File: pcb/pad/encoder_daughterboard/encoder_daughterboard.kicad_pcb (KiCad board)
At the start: 2 copper layers, 91.4 x 26.9 mm, 9 parts, among them J1 Conn_01x12, SW1 RotaryEncoder_Switch_MP, SW2 RotaryEncoder_Switch_MP, SW3 RotaryEncoder_Switch_MP

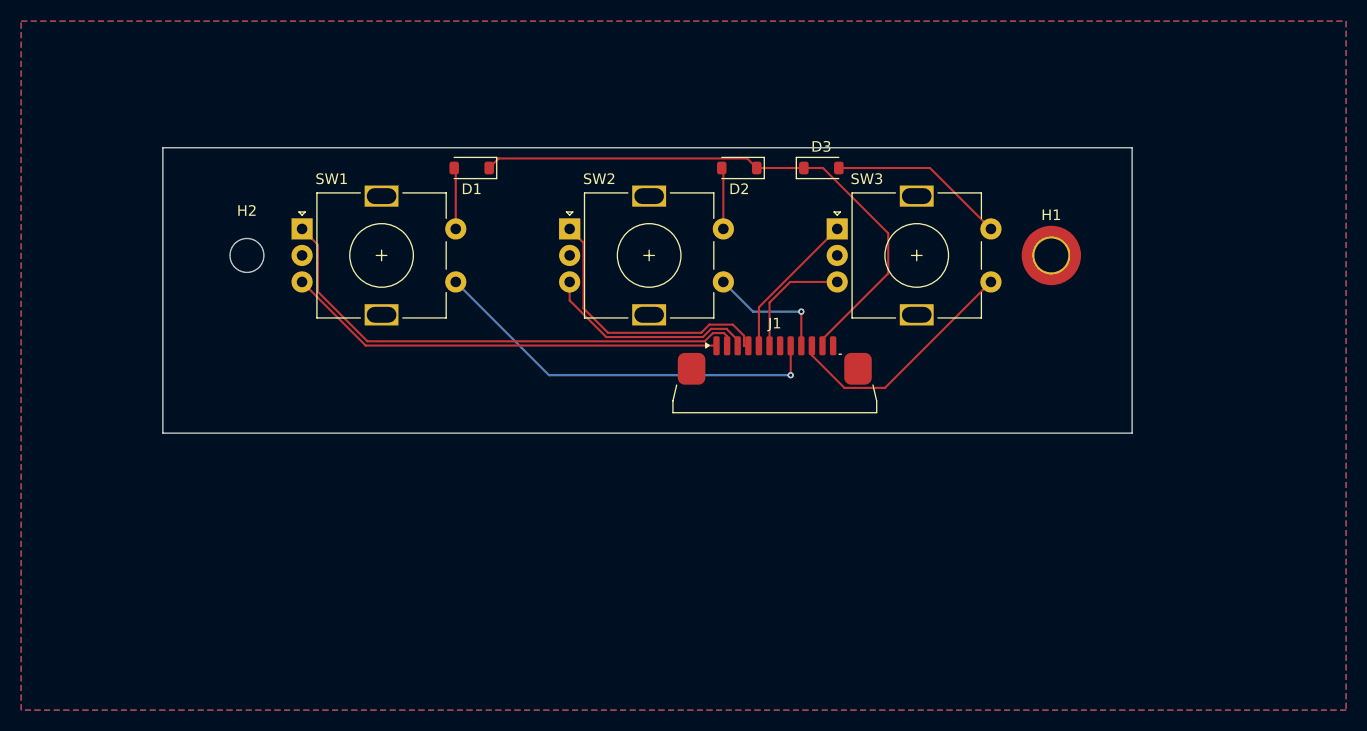
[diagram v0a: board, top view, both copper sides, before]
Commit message: Update encoder_daughterboard
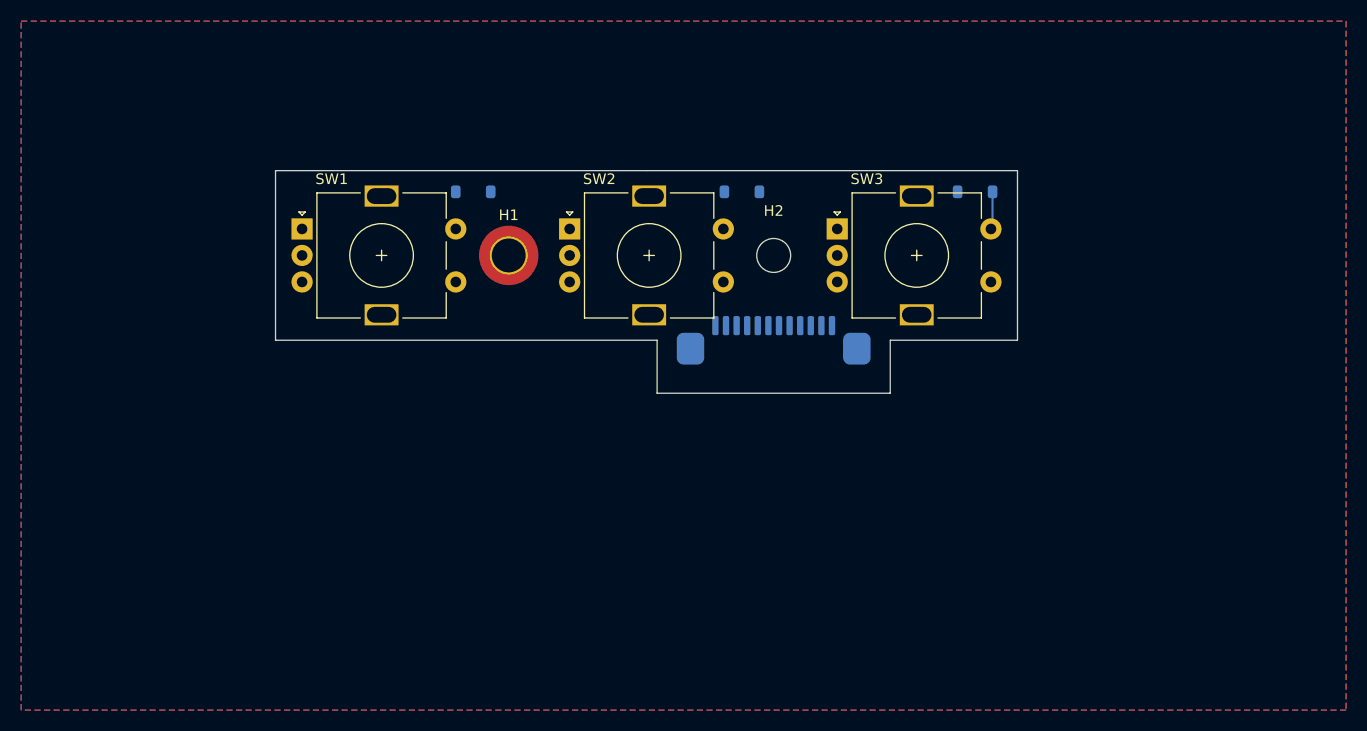
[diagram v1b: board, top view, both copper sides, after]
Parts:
- D1, D2, D3: moved to B.Cu
- J1: value Conn_01x12 -> AFA07-S12FCA-00; moved to B.Cu
- SW1, SW2, SW3: value RotaryEncoder_Switch_MP -> EC11E09244BS
- moved H1 51.2 mm to (95.2, 78.2)
- moved H2 49.7 mm to (120.2, 78.2)
- moved D3 14.7 mm to (139.2, 72.2)
- moved D2 2.26 mm to (117.2, 72.2)
- moved D1 2.25 mm to (91.9, 72.2)
- moved J1 1.90 mm to (120.2, 88.2), turned to 180 degrees
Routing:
- net BRow0: track 54.1 -> 0.00 mm
- net E0A: track 48.4 -> 0.00 mm
- net E0B: track 41.6 -> 0.00 mm
- net BCol0: track 38.0 -> 0.00 mm, vias 1 -> 0
- net E1A: track 26.2 -> 0.00 mm
- net BCol2: track 23.2 -> 0.00 mm
- net E1B: track 20.3 -> 0.00 mm
- net E2A: track 14.1 -> 0.00 mm
- net Net-(D3-A): track 16.7 -> 3.56 mm
- net BCol1: track 11.7 -> 0.00 mm, vias 1 -> 0
- net E2B: track 11.3 -> 0.00 mm
- net Net-(D2-A): track 5.81 -> 0.00 mm
- net Net-(D1-A): track 5.81 -> 0.00 mm
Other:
- board size 91.4 x 26.9 mm -> 70 x 21 mm

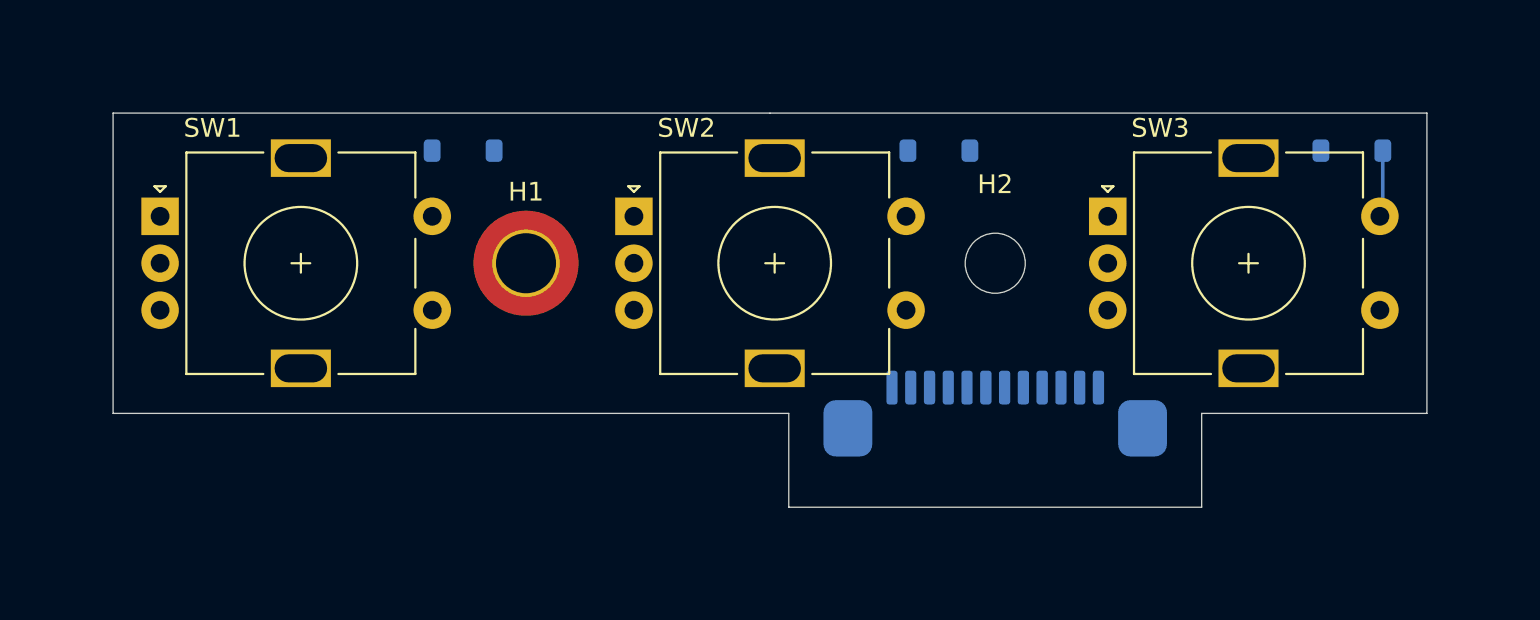
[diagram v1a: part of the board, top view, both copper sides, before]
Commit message: Update encoder_daughterboard
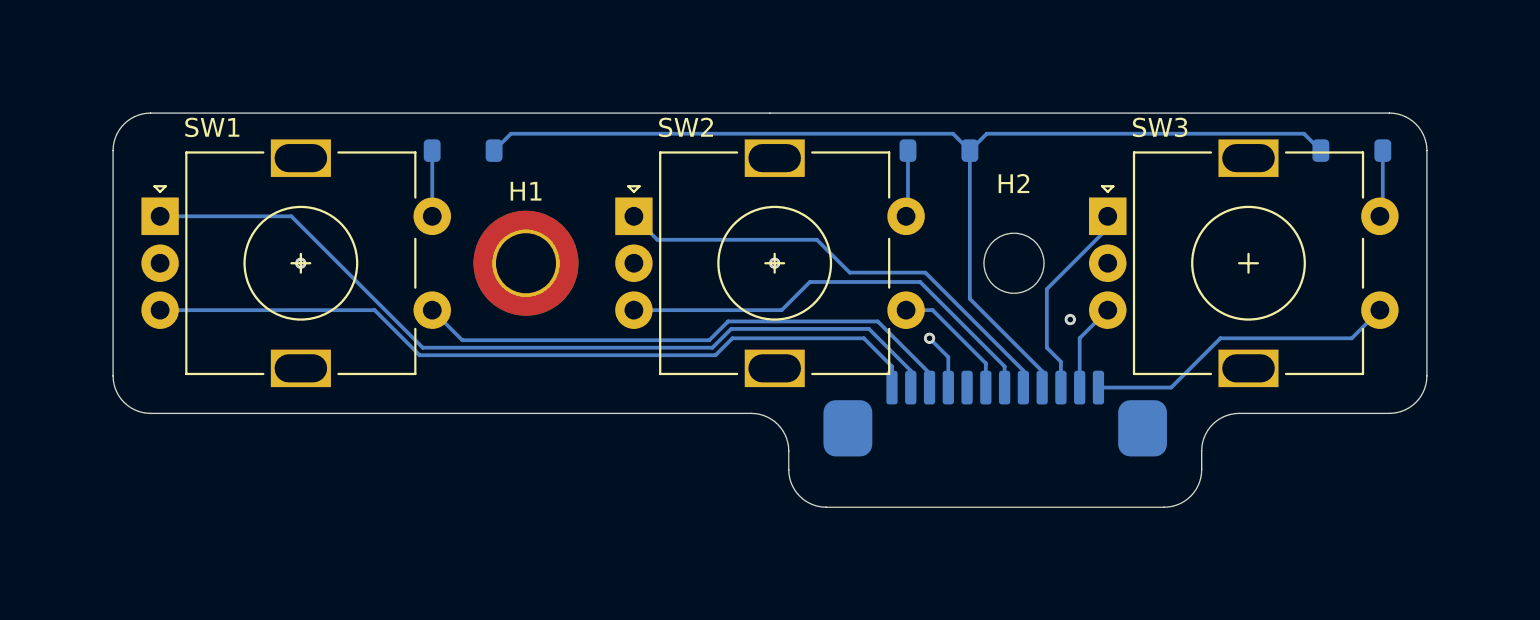
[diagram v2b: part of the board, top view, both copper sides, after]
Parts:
- H1: value MountingHole_Pad_MP -> MountingHole_Pad
- moved H2 1.00 mm to (121.2, 78.2)
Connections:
- H1 pad 1: (no net) -> GND
- J1 pad 1: E0B -> BCol2
- J1 pad 10: BCol2 -> BCol0
- J1 pad 11: BRow0 -> E0A
- J1 pad 12: GND -> E0B
- J1 pad 2: E0A -> E2B
- J1 pad 3: E1B -> E2A
- J1 pad 4: E1A -> BRow0
- J1 pad 5: E2A -> E1A
- J1 pad 6: E2B -> E1B
- J1 pad 7: GND -> BCol1
- J1 pad 8: BCol0 -> GND
- J1 pad 9: BCol1 -> GND
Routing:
- net BRow0: track 0.00 -> 59.8 mm
- net E0A: track 0.00 -> 45.1 mm
- net E0B: track 0.00 -> 42.1 mm
- net BCol0: track 0.00 -> 29.5 mm
- net E1A: track 0.00 -> 25.1 mm
- net E1B: track 0.00 -> 23.7 mm
- net BCol2: track 0.00 -> 16.7 mm
- net E2A: track 0.00 -> 10.8 mm
- net BCol1: track 0.00 -> 6.71 mm
- net E2B: track 0.00 -> 4.74 mm
- net Net-(D2-A): track 0.00 -> 3.54 mm
- net Net-(D1-A): track 0.00 -> 3.50 mm
- net GND: track 0.00 -> 3.04 mm, vias 0 -> 4
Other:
- outline, holes or cut-outs redrawn
